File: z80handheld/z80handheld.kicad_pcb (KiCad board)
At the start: 4 copper layers, 102.2 x 147.6 mm, 137 parts, among them IC1 DS12885+, J1 Power, J2 Esp32 C3 Supermini Right, J3 SPI Screen, J4 Esp32 C3 Supermini Left, SW1 SW_Push_45deg, SW10 SW_Push_45deg, SW11 SW_Push_45deg, SW12 SW_Push_45deg, SW13 SW_Push_45deg, SW14 SW_Push_45deg, SW15 SW_Push_45deg, SW16 SW_Push_45deg, SW17 SW_Push_45deg, SW18 SW_Push_45deg, SW19 SW_Push_45deg, SW2 SW_Push_45deg, SW20 SW_Push_45deg, SW21 SW_Push_45deg, SW22 SW_Push_45deg, SW23 SW_Push_45deg, SW24 SW_Push_45deg, SW25 SW_Push_45deg, SW26 SW_Push_45deg, SW27 SW_Push_45deg, SW28 SW_Push_45deg, SW29 SW_Push_45deg, SW3 SW_Push_45deg, SW30 SW_Push_45deg, SW31 SW_Push_45deg, SW32 SW_Push_45deg, SW33 SW_Push_45deg, SW34 SW_Push_45deg, SW35 SW_Push_45deg, SW36 SW_Push_45deg, SW37 SW_Push_45deg, SW38 SW_Push_45deg, SW39 SW_Push_45deg, SW4 SW_Push_45deg, SW40 SW_Push_45deg, SW41 SW_Push_45deg, SW42 SW_Push_45deg, SW43 SW_Push_45deg, SW44 SW_Push_45deg, SW45 SW_Push_45deg, SW46 SW_Push_45deg, SW47 SW_Push_45deg, SW48 SW_Push_45deg, SW49 SW_Push_45deg, SW5 SW_Push_45deg, SW50 SW_Push_45deg, SW51 SW_Push_45deg, SW52 SW_Push_45deg, SW53 SW_Push_45deg, SW54 SW_Push_45deg, SW55 SW_Push_45deg, SW56 SW_Push_45deg, SW57 SW_Push_45deg, SW58 SW_Push_45deg, SW59 SW_Push_45deg, SW6 SW_Push_45deg, SW60 SW_Push_45deg, SW61 SW_Push_45deg, SW62 SW_Push_45deg, SW63 SW_Push_45deg, SW64 SW_Push_45deg, SW65 SW_Push, SW7 SW_Push_45deg, SW8 SW_Push_45deg, SW9 SW_Push_45deg, U1 74HC04, U10 Z84C00xxP, U11 74LS573 IO1, U12 HDSP-7501, U13 74LS573, U14 HDSP-7501, U15 74LS573, U16 16550 IO2, U17 16550 IO3, U2 4068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

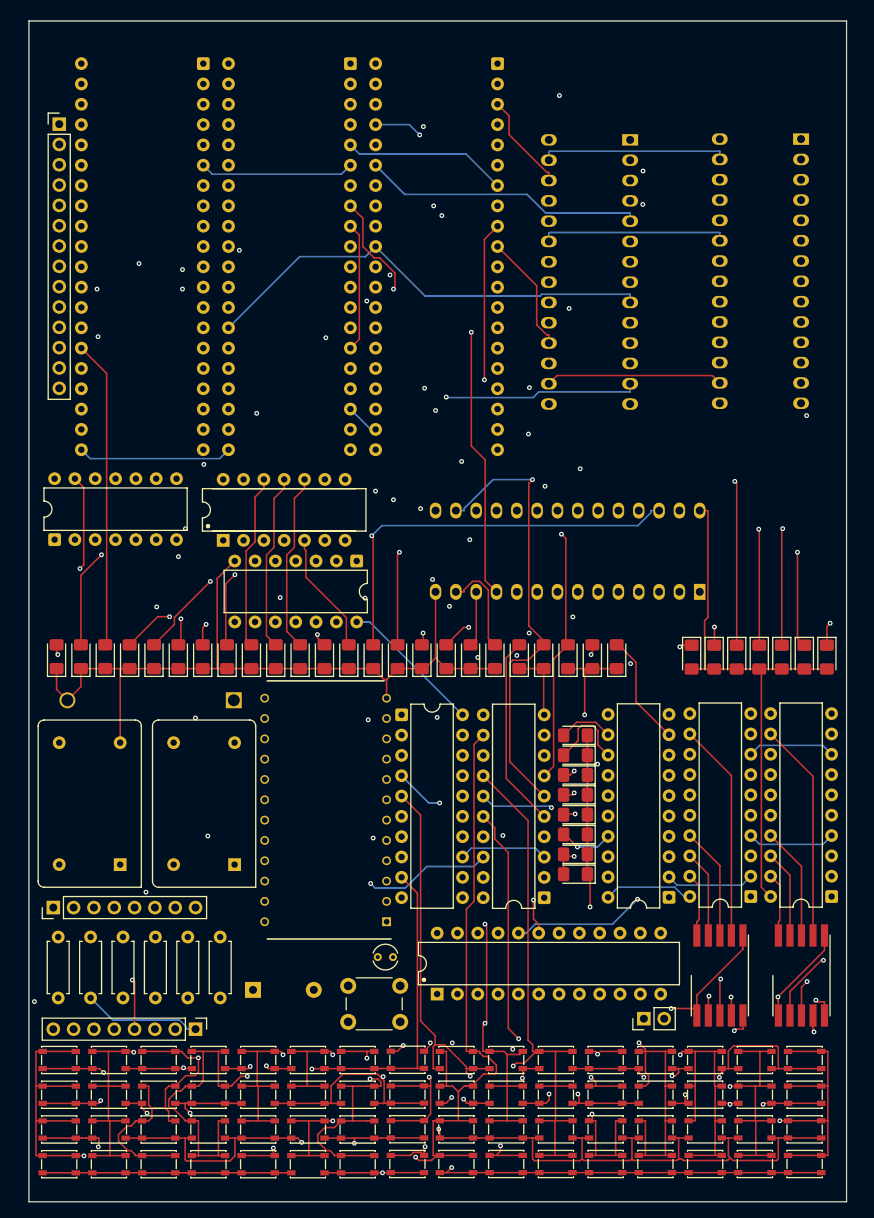
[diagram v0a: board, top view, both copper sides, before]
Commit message: Add files via upload
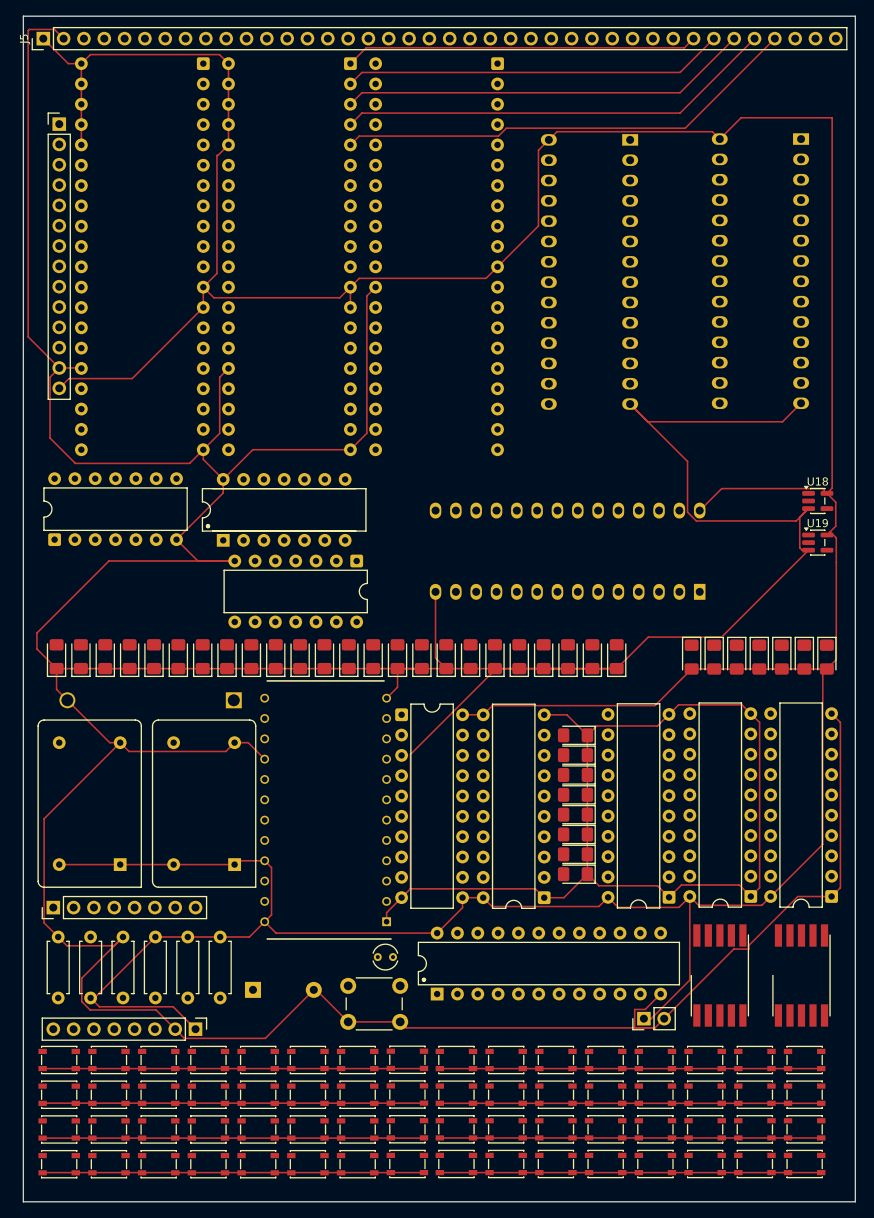
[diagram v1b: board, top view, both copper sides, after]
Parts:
- added J5: Conn_01x40, Connector_PinHeader_2.54mm:PinHeader_1x40_P2.54mm_Vertical, F.Cu at (208.4, 70.1)
- added U18: 74AHCT1G32, Package_TO_SOT_SMD:SC-74A-5_1.55x2.9mm_P0.95mm, F.Cu at (305.2, 127.9)
- added U19: 74AHCT1G32, Package_TO_SOT_SMD:SC-74A-5_1.55x2.9mm_P0.95mm, F.Cu at (305.2, 133.1)
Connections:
- net Net-(U10-CLK) renamed CLK
- D3 pad 2: !MREQ -> BANK_0
- D31 pad 2: !MREQ -> A15
- U1 pad 12: !MREQ -> Net-(U7-~{CS})
- U1 pad 13: !MREQ -> A15
- U1 pad 3: !MREQ -> A15
- U10 pad 5: !MREQ -> A15
- U2 pad 2: !MREQ -> A15
- U3 pad 8: unconnected-(U3-Pad8) -> IO8
- U3 pad 9: unconnected-(U3-Pad9) -> IO1
- U6 pad 19: !MREQ -> BANK_0
- U7 pad 20: !MREQ -> Net-(U7-~{CS})
- U9 pad 20: !MREQ -> Net-(U9-~{CS})
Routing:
- net D2: track 300.1 -> 51.4 mm, vias 2 -> 0
- net A7: track 232.3 -> 0.00 mm, vias 3 -> 0
- net D6: track 224.5 -> 0.00 mm, vias 2 -> 0
- net A0: track 223.1 -> 0.00 mm, vias 3 -> 0
- net !WR: track 219.9 -> 0.00 mm, vias 2 -> 0
- net A5: track 214.8 -> 0.00 mm, vias 2 -> 0
- net A6: track 214.6 -> 0.00 mm, vias 3 -> 0
- net D5: track 214.2 -> 0.00 mm, vias 2 -> 0
- net A4: track 210.4 -> 0.00 mm, vias 3 -> 0
- net !MREQ: track 210.3 -> 0.00 mm, vias 5 -> 0
- net !RD: track 207.7 -> 0.00 mm, vias 2 -> 0
- net D7: track 206.2 -> 0.00 mm, vias 1 -> 0
- net D1: track 251.3 -> 47.8 mm, vias 1 -> 0
- net GND: track 560.1 -> 763.2 mm, vias 2 -> 0
- net D0: track 245.8 -> 44.2 mm, vias 3 -> 0
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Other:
- board size 102.2 x 147.6 mm -> 104 x 148.2 mm

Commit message: Add files via upload
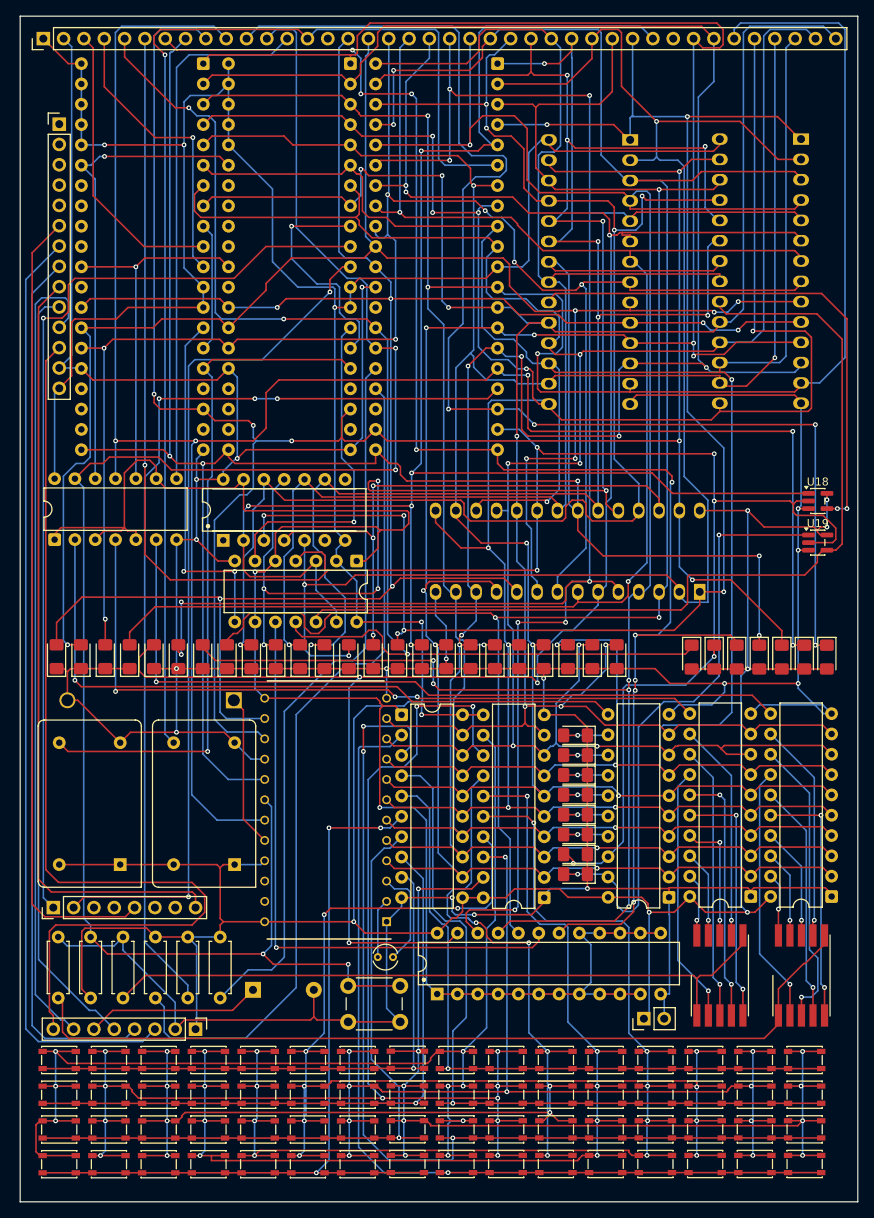
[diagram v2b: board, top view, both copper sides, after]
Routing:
- net D5: track 0.00 -> 312.4 mm, vias 0 -> 4
- net D6: track 0.00 -> 281.5 mm, vias 0 -> 6
- net D7: track 0.00 -> 267.6 mm, vias 0 -> 7
- net D2: track 51.4 -> 316.9 mm, vias 0 -> 5
- net !RD: track 0.00 -> 264.5 mm, vias 0 -> 5
- net D0: track 44.2 -> 307.5 mm, vias 0 -> 7
- net !WR: track 0.00 -> 262.3 mm, vias 0 -> 6
- net !MREQ: track 0.00 -> 258.0 mm, vias 0 -> 7
- net A5: track 0.00 -> 256.1 mm, vias 0 -> 9
- net D1: track 47.8 -> 300.3 mm, vias 0 -> 7
- net !INT: track 0.00 -> 251.8 mm, vias 0 -> 5
- net A0: track 0.00 -> 250.3 mm, vias 0 -> 6
- net A6: track 0.00 -> 248.5 mm, vias 0 -> 6
- net D3: track 55.0 -> 298.2 mm, vias 0 -> 9
- net A4: track 0.00 -> 242.9 mm, vias 0 -> 6
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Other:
- board size 104 x 148.2 mm -> 104.7 x 148.2 mm
- copper layers 4 -> 2
